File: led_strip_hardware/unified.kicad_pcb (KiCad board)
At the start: 4 copper layers, 48.3 x 20.3 mm, 36 parts, among them P1 mod_jack_in, P2 PWR_TST, P3 LED_STRIP, P4 ICSP, Q1 FDN5618P, SW1 USR_SW, U1 ISL83485IBZ, U2 TPS54560, U3 STM32F030-32, U4 NCP1117ST33T3G, U5 2CH-TVS

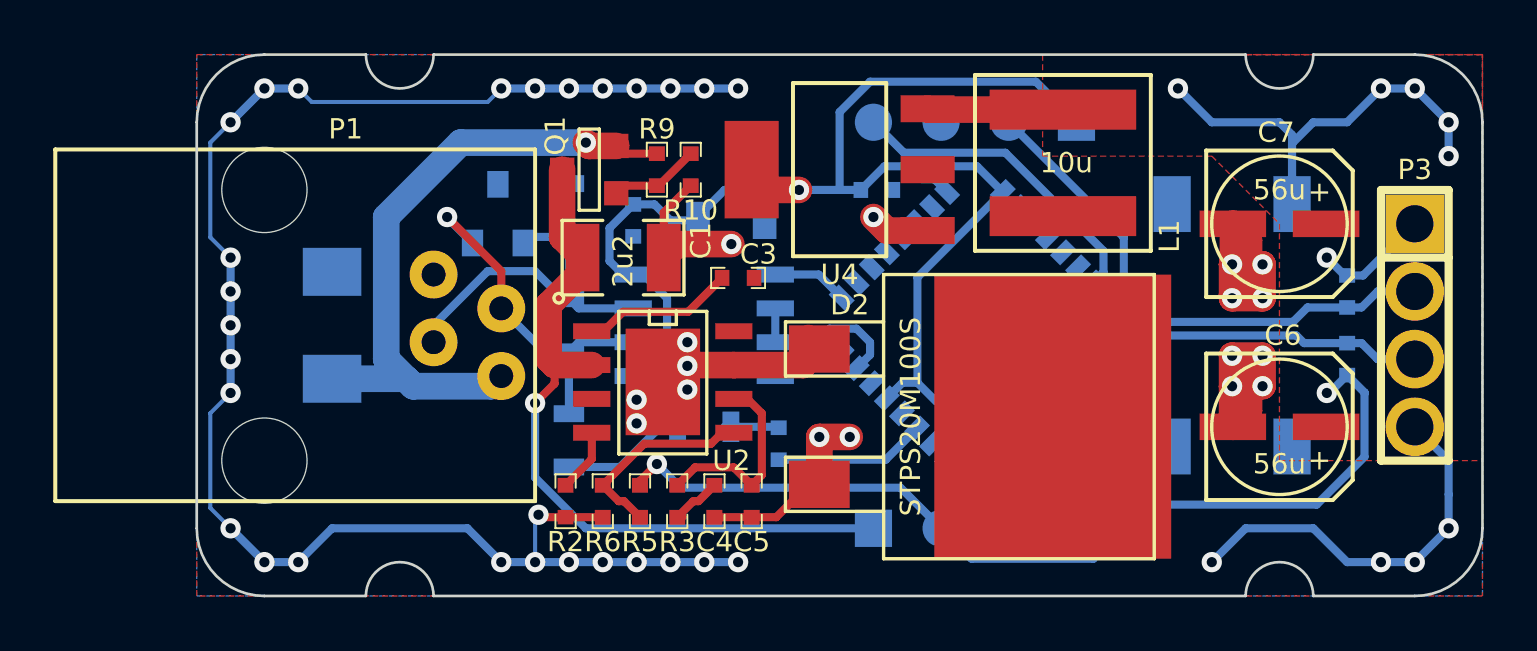
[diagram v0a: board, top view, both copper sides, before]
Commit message: Progress on v7 of led_strip_hardware
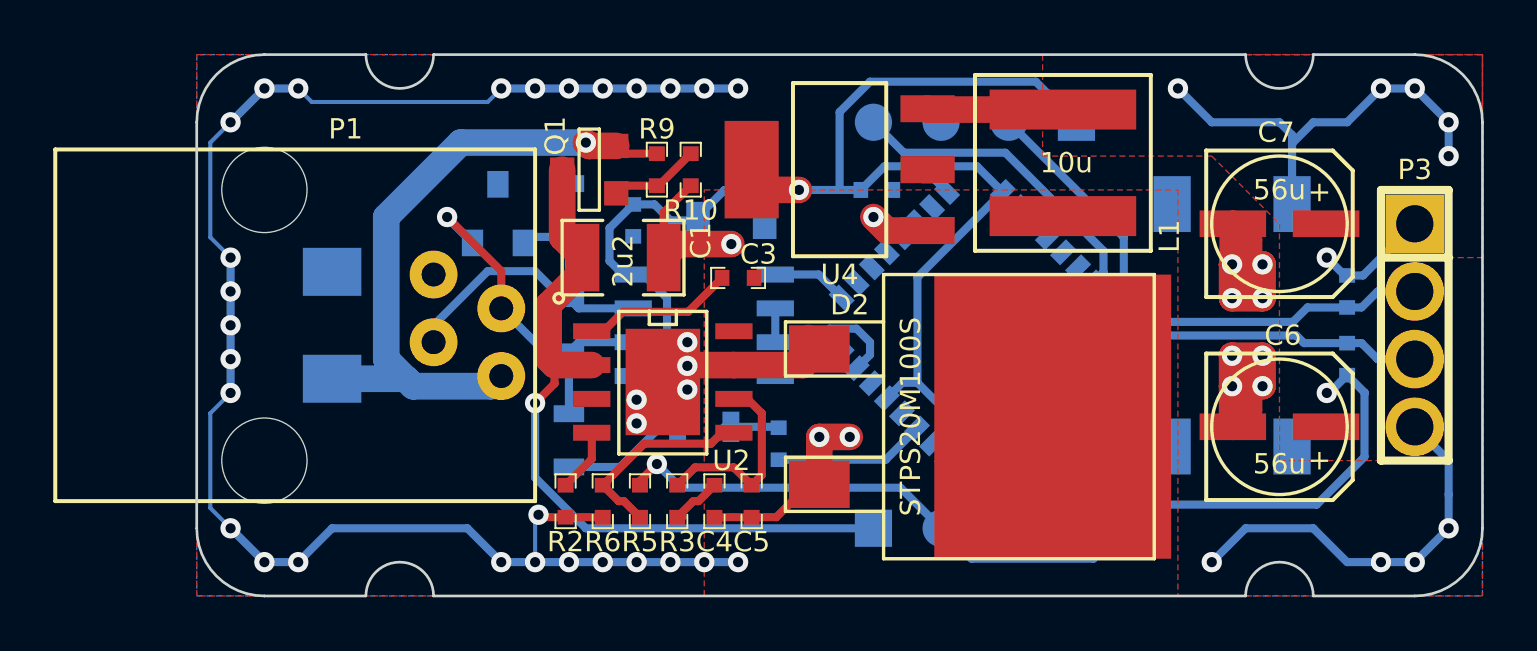
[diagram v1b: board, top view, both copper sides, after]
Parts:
- R5: value 68K -> 270K
- R6: value 12K -> 22K
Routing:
- added copper zone on F.Cu, net GND
